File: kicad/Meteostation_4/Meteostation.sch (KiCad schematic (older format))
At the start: 106 parts, among them J1 TxD, J10 GM+, J11 GM-, J12 SWD, J13 SWC, J2 RxD, J3 BME280_SCL, J4 BME280_SDA, J6 +EXT, J7 -EXT, Q1 5N10, Q2 IRLML6346, Q3 Q_NPN_BEC, T1 HY931147C, U1 STM32F103C8Tx, U2 LMR14206, U3 AD8541, Y2 ECS-250-20-33 25MHz

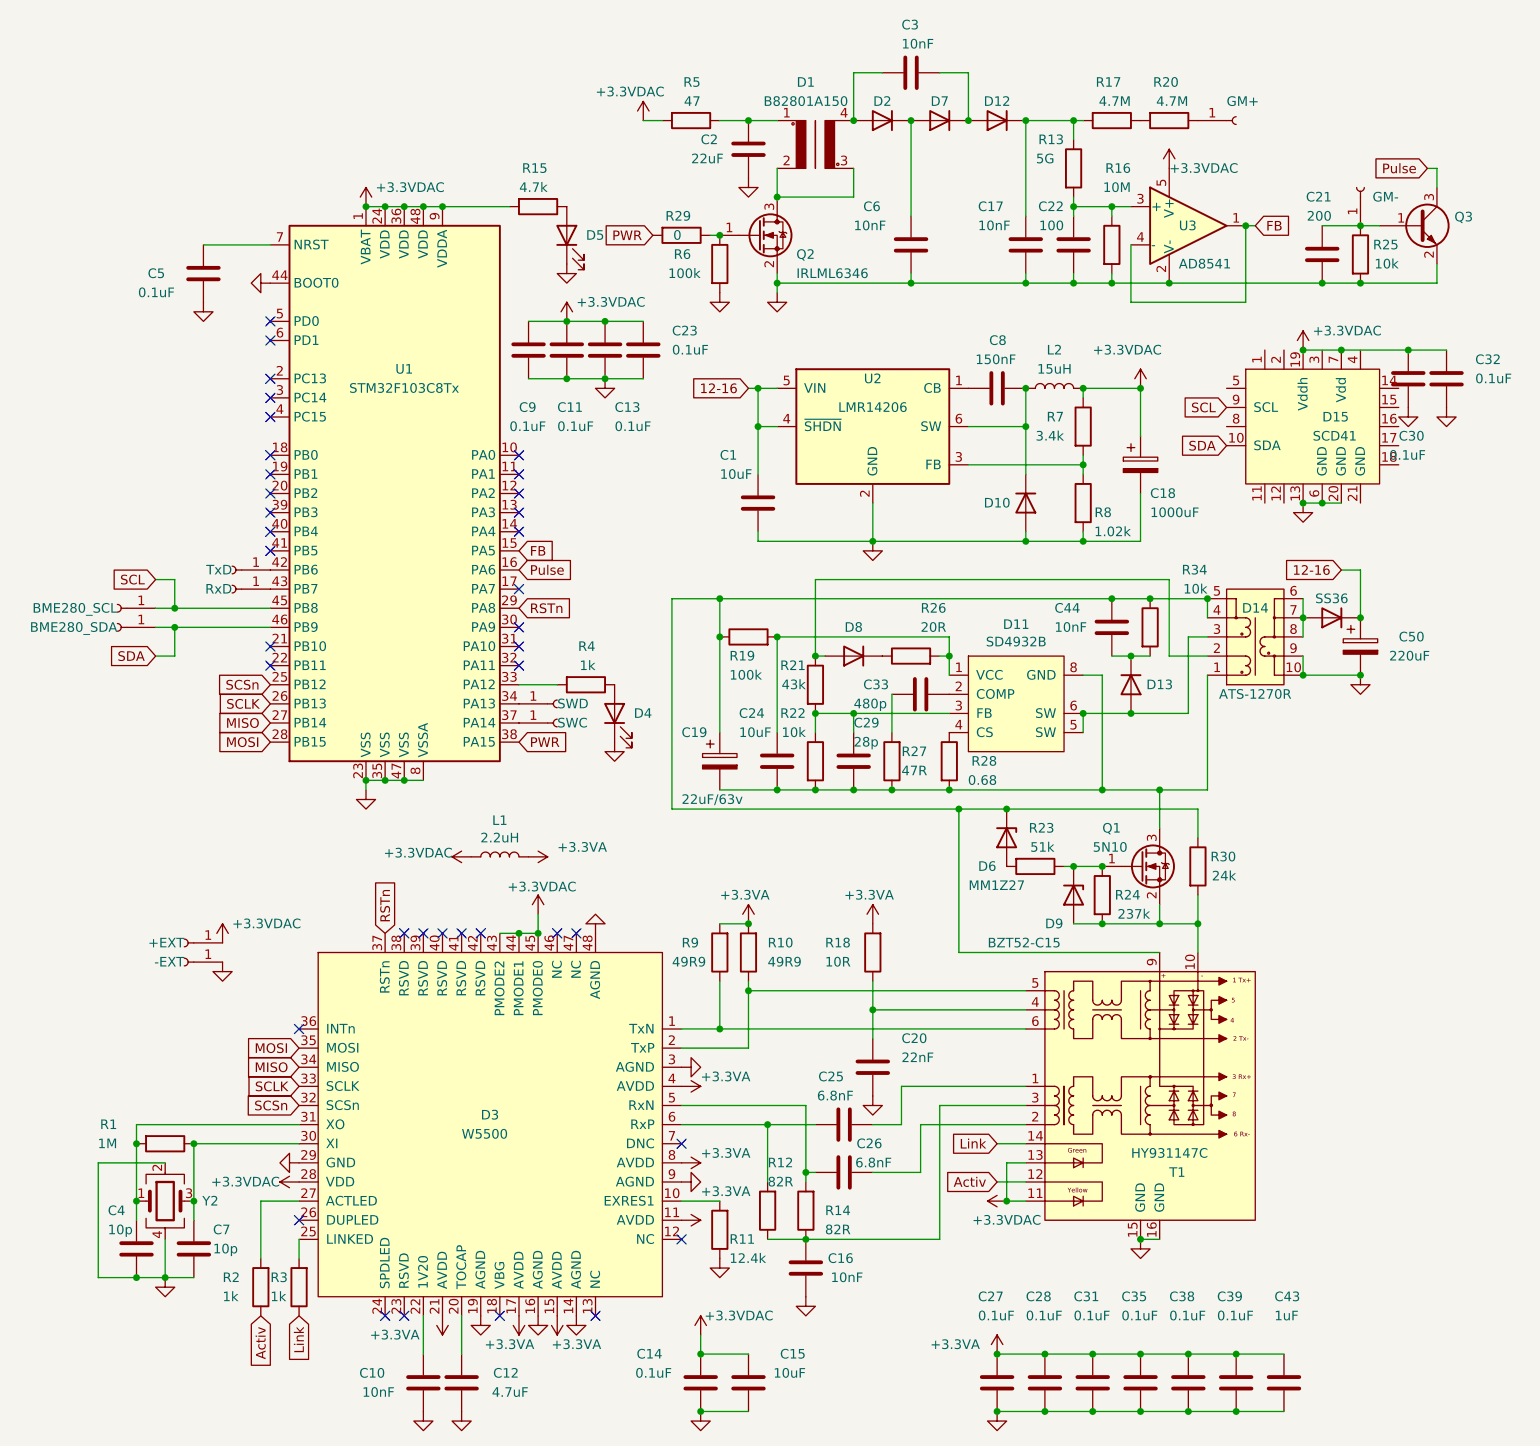
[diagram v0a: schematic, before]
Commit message: изменено:      kicad/Meteostation_4/Meteostation.kicad_pcb 	изменено:      kicad/Meteostation_4/Meteostation.kicad_pcb-bak 	изменено:      kicad/Meteostation_4/Meteostation.sch 	изменено:      kicad/Meteostation_4/Meteostation.sch-bak 	изменено:      kicad/Meteostation_4/fp-info-cache 	изменено:      kicad/Meteostation_4/gerber/Meteostation-job.gbrjob
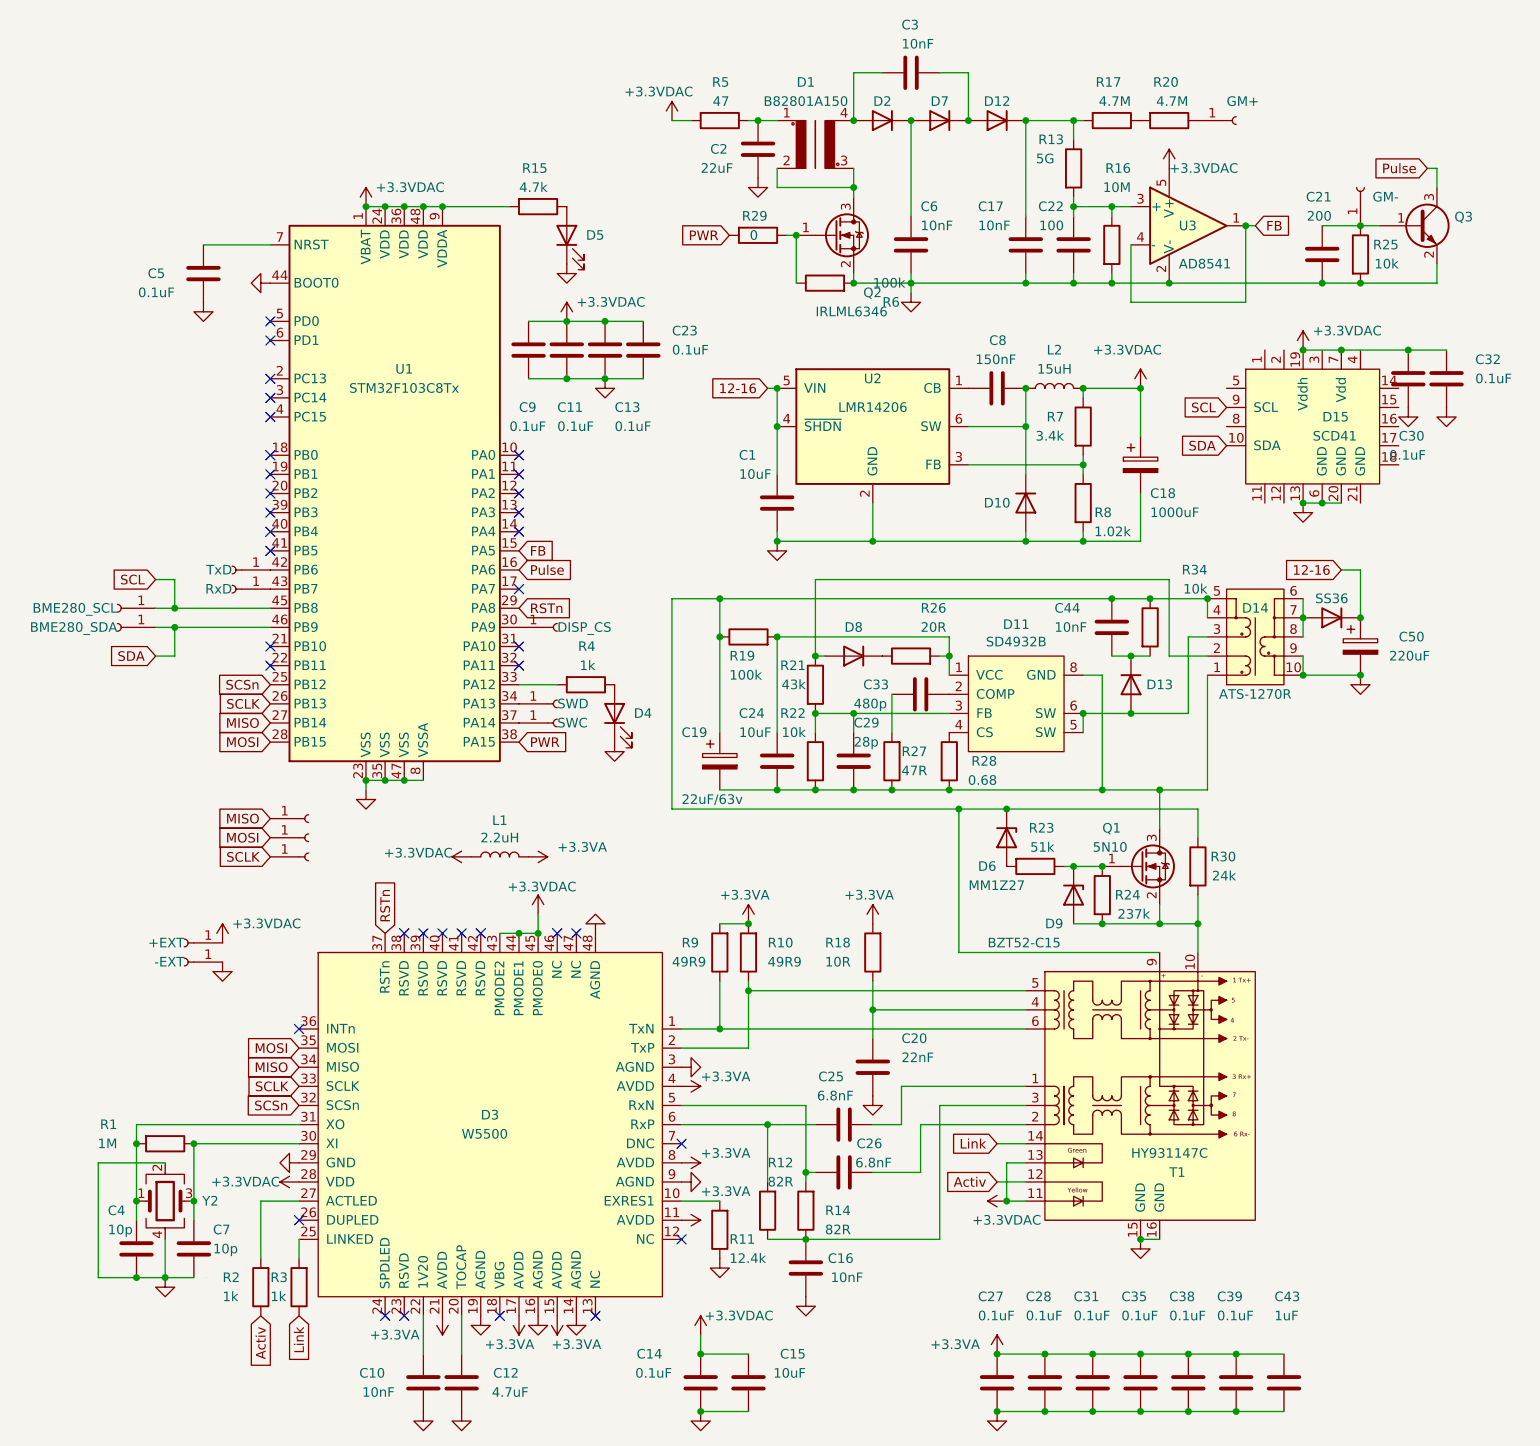
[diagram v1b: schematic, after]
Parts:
- added J14: DISP_CS, My-library:ConnMini, symbol Connector:Conn_01x01_Female
- added J5: miso, My-library:ConnMini, symbol Connector:Conn_01x01_Female
- added J8: mosi, My-library:ConnMini, symbol Connector:Conn_01x01_Female
- added J9: sclk, My-library:ConnMini, symbol Connector:Conn_01x01_Female
- R4: footprint Resistor_SMD:R_0603_1608Metric -> Resistor_SMD:R_0402_1005Metric
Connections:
- net MISO: now also J5.1 (Pin_1)
- net MOSI: now also J8.1 (Pin_1)
- net SCLK: now also J9.1 (Pin_1)
- net at U1.30 (PA9): now also J14.1 (Pin_1)
- no-connect marks 37 -> 36
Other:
- moved on the sheet: C1, C2, Q2, R29, R5, R6
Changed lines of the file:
@@
 F 0 "R4" V 6300 5700 50  0000 R CNN
 F 1 "1k" V 6400 5700 50  0000 R CNN
-F 2 "Resistor_SMD:R_0603_1608Metric" V 6430 5650 50  0001 C CNN
+F 2 "Resistor_SMD:R_0402_1005Metric" V 6430 5650 50  0001 C CNN
 F 3 "~" H 6500 5650 50  0001 C CNN
 	1    6500 5650
@@
 	1    0    0    -1
 $EndComp
-Text GLabel 7350 4100 0    50   Input ~ 0
+Text GLabel 7450 4100 0    50   Input ~ 0
 12-16
 $Comp
@@
 L power:GND #PWR029
 U 1 1 63349FA6
-P 8000 4900
-F 0 "#PWR029" H 8000 4650 50  0001 C CNN
-F 1 "GND" H 8005 4727 50  0001 C CNN
-F 2 "" H 8000 4900 50  0001 C CNN
-F 3 "" H 8000 4900 50  0001 C CNN
-	1    8000 4900
+P 7500 4900
+F 0 "#PWR029" H 7500 4650 50  0001 C CNN
+F 1 "GND" H 7505 4727 50  0001 C CNN
+F 2 "" H 7500 4900 50  0001 C CNN
+F 3 "" H 7500 4900 50  0001 C CNN
+	1    7500 4900
 	1    0    0    -1
 $EndComp
@@
 L Device:C C1
 U 1 1 634777B2
-P 7400 4700
-F 0 "C1" H 7200 4950 50  0000 L CNN
-F 1 "10uF" H 7200 4850 50  0000 L CNN
-F 2 "Capacitor_SMD:C_0805_2012Metric" H 7438 4550 50  0001 C CNN
-F 3 "~" H 7400 4700 50  0001 C CNN
-	1    7400 4700
-	1    0    0    -1
-$EndComp
-Wire Wire Line
-	7400 4100 7500 4100
-Wire Wire Line
-	7500 4300 7400 4300
-Wire Wire Line
-	7400 4300 7400 4100
-Wire Wire Line
-	7400 4300 7400 4550
-Connection ~ 7400 4300
-Wire Wire Line
-	8000 4900 7400 4900
-Wire Wire Line
-	7400 4900 7400 4850
+P 7500 4700
+F 0 "C1" H 7300 4950 50  0000 L CNN
+F 1 "10uF" H 7300 4850 50  0000 L CNN
+F 2 "Capacitor_SMD:C_0805_2012Metric" H 7538 4550 50  0001 C CNN
+F 3 "~" H 7500 4700 50  0001 C CNN
+	1    7500 4700
+	1    0    0    -1
+$EndComp
 $Comp
 L power:GND #PWR013
@@
 $EndComp
 $Comp
-L Transistor_FET:BSS138 Q2
-U 1 1 6364CAE8
-P 7400 3300
-F 0 "Q2" H 7600 3200 50  0000 L CNN
-F 1 "IRLML6346" H 7600 3100 50  0000 L CNN
-F 2 "Package_TO_SOT_SMD:SOT-23" H 7600 3225 50  0001 L CIN
-F 3 "https://www.onsemi.com/pub/Collateral/BSS138-D.PDF" H 7400 3300 50  0001 L CNN
-	1    7400 3300
-	1    0    0    -1
-$EndComp
-$Comp
 L Meteostation-rescue:B82801A1-My_Library D1
 U 1 1 6364FE98
@@
 $EndComp
 Wire Wire Line
-	7500 2950 7500 3100
-Wire Wire Line
-	7500 3100 7900 3100
-Wire Wire Line
-	7900 3100 7900 2950
-Connection ~ 7500 3100
+	7900 3100 7900 3050
 $Comp
 L power:GND #PWR028
 U 1 1 63678BE2
-P 7500 3600
-F 0 "#PWR028" H 7500 3350 50  0001 C CNN
-F 1 "GND" H 7505 3427 50  0001 C CNN
-F 2 "" H 7500 3600 50  0001 C CNN
-F 3 "" H 7500 3600 50  0001 C CNN
-	1    7500 3600
+P 8200 3600
+F 0 "#PWR028" H 8200 3350 50  0001 C CNN
+F 1 "GND" H 8205 3427 50  0001 C CNN
+F 2 "" H 8200 3600 50  0001 C CNN
+F 3 "" H 8200 3600 50  0001 C CNN
+	1    8200 3600
 	1    0    0    -1
 $EndComp
@@
 U 1 1 636874B8
 P 8200 3350
-F 0 "C6" H 7950 3550 50  0000 L CNN
-F 1 "10nF" H 7900 3450 50  0000 L CNN
+F 0 "C6" H 8250 3550 50  0000 L CNN
+F 1 "10nF" H 8250 3450 50  0000 L CNN
 F 2 "Capacitor_SMD:C_1206_3216Metric" H 8238 3200 50  0001 C CNN
 F 3 "~" H 8200 3350 50  0001 C CNN
@@
 $EndComp
 Wire Wire Line
-	7500 3550 7500 3500
-Wire Wire Line
-	7500 3550 7500 3600
-Connection ~ 7500 3550
-Text GLabel 6850 3300 0    50   Input ~ 0
-PWR
+	8200 3550 8200 3600
 $Comp
 L Device:C C2
 U 1 1 63742F99
-P 7350 2850
-F 0 "C2" H 7100 2900 50  0000 L CNN
-F 1 "22uF" H 7050 2800 50  0000 L CNN
-F 2 "Capacitor_SMD:C_0805_2012Metric" H 7388 2700 50  0001 C CNN
-F 3 "~" H 7350 2850 50  0001 C CNN
-	1    7350 2850
-	1    0    0    -1
-$EndComp
-Wire Wire Line
-	7500 2700 7350 2700
+P 7400 2850
+F 0 "C2" H 7150 2850 50  0000 L CNN
+F 1 "22uF" H 7100 2750 50  0000 L CNN
+F 2 "Capacitor_SMD:C_0805_2012Metric" H 7438 2700 50  0001 C CNN
+F 3 "~" H 7400 2850 50  0001 C CNN
+	1    7400 2850
+	1    0    0    -1
+$EndComp
+Wire Wire Line
+	7500 2700 7400 2700
 $Comp
 L power:GND #PWR027
 U 1 1 6374F84D
-P 7350 3000
-F 0 "#PWR027" H 7350 2750 50  0001 C CNN
-F 1 "GND" H 7355 2827 50  0001 C CNN
-F 2 "" H 7350 3000 50  0001 C CNN
-F 3 "" H 7350 3000 50  0001 C CNN
-	1    7350 3000
+P 7400 3000
+F 0 "#PWR027" H 7400 2750 50  0001 C CNN
+F 1 "GND" H 7405 2827 50  0001 C CNN
+F 2 "" H 7400 3000 50  0001 C CNN
+F 3 "" H 7400 3000 50  0001 C CNN
+	1    7400 3000
 	1    0    0    -1
 $EndComp
@@
 L Device:R R5
 U 1 1 63751028
-P 7050 2700
-F 0 "R5" V 6850 2750 50  0000 R CNN
-F 1 "47" V 6950 2750 50  0000 R CNN
-F 2 "Resistor_SMD:R_1206_3216Metric" V 6980 2700 50  0001 C CNN
-F 3 "~" H 7050 2700 50  0001 C CNN
-	1    7050 2700
+P 7200 2700
+F 0 "R5" V 7000 2750 50  0000 R CNN
+F 1 "47" V 7100 2750 50  0000 R CNN
+F 2 "Resistor_SMD:R_1206_3216Metric" V 7130 2700 50  0001 C CNN
+F 3 "~" H 7200 2700 50  0001 C CNN
+	1    7200 2700
 	0    1    1    0
 $EndComp
@@
 L power:+3.3VDAC #PWR023
 U 1 1 63754194
-P 6800 2700
-F 0 "#PWR023" H 6950 2650 50  0001 C CNN
-F 1 "+3.3VDAC" H 6550 2850 50  0000 L CNN
-F 2 "" H 6800 2700 50  0001 C CNN
-F 3 "" H 6800 2700 50  0001 C CNN
-	1    6800 2700
-	1    0    0    -1
-$EndComp
-Wire Wire Line
-	6800 2700 6900 2700
+P 6950 2700
+F 0 "#PWR023" H 7100 2650 50  0001 C CNN
+F 1 "+3.3VDAC" H 6700 2850 50  0000 L CNN
+F 2 "" H 6950 2700 50  0001 C CNN
+F 3 "" H 6950 2700 50  0001 C CNN
+	1    6950 2700
+	1    0    0    -1
+$EndComp
+Wire Wire Line
+	6950 2700 7050 2700
 $Comp
 L Device:R R17
@@
 NoConn ~ 4850 4950
 NoConn ~ 6150 5150
-NoConn ~ 6150 5350
 NoConn ~ 6150 5450
 NoConn ~ 6150 5550
@@
 	10950 3450 10950 3550
 Wire Wire Line
-	7350 4100 7400 4100
-Connection ~ 7400 4100
-Wire Wire Line
 	10900 2950 10950 2950
 Wire Wire Line
@@
 Wire Wire Line
 	9250 3200 9250 3150
-Wire Wire Line
-	7500 3550 8200 3550
 Connection ~ 9250 3150
 Wire Wire Line
@@
 Wire Wire Line
 	8200 3550 8800 3550
-Connection ~ 7350 2700
-Wire Wire Line
-	7350 2700 7200 2700
 Wire Wire Line
 	7650 7850 7650 8200
@@
 	7700 5100 9550 5100
 $Comp
-L Device:R R6
-U 1 1 634FB19F
-P 7200 3450
-F 0 "R6" H 7050 3500 50  0000 R CNN
-F 1 "100k" H 7100 3400 50  0000 R CNN
-F 2 "Resistor_SMD:R_0603_1608Metric" V 7130 3450 50  0001 C CNN
-F 3 "~" H 7200 3450 50  0001 C CNN
-	1    7200 3450
-	1    0    0    -1
-$EndComp
-$Comp
-L power:GND #PWR043
-U 1 1 63505702
-P 7200 3600
-F 0 "#PWR043" H 7200 3350 50  0001 C CNN
-F 1 "GND" H 7205 3427 50  0001 C CNN
-F 2 "" H 7200 3600 50  0001 C CNN
-F 3 "" H 7200 3600 50  0001 C CNN
-	1    7200 3600
-	1    0    0    -1
-$EndComp
-$Comp
 L Device:R R16
 U 1 1 636A0C6A
@@
 Wire Wire Line
 	10800 3900 11000 3900
+Wire Wire Line
+	7550 3300 7600 3300
 $Comp
 L Device:R R29
 U 1 1 635E067E
-P 7000 3300
-F 0 "R29" V 6900 3350 50  0000 R CNN
-F 1 "0" V 7000 3300 50  0000 R CNN
-F 2 "Resistor_SMD:R_1206_3216Metric" V 6930 3300 50  0001 C CNN
-F 3 "~" H 7000 3300 50  0001 C CNN
-	1    7000 3300
+P 7400 3300
+F 0 "R29" V 7300 3350 50  0000 R CNN
+F 1 "0" V 7400 3300 50  0000 R CNN
+F 2 "Resistor_SMD:R_1206_3216Metric" V 7330 3300 50  0001 C CNN
+F 3 "~" H 7400 3300 50  0001 C CNN
+	1    7400 3300
 	0    1    1    0
 $EndComp
-Wire Wire Line
-	7150 3300 7200 3300
-Connection ~ 7200 3300
+$Comp
+L Device:R R6
+U 1 1 634FB19F
+P 7750 3550
+F 0 "R6" V 7650 3250 50  0000 R CNN
+F 1 "100k" V 7750 3300 50  0000 R CNN
+F 2 "Resistor_SMD:R_0603_1608Metric" V 7680 3550 50  0001 C CNN
+F 3 "~" H 7750 3550 50  0001 C CNN
+	1    7750 3550
+	0    -1   -1   0
+$EndComp
+Text GLabel 7250 3300 0    50   Input ~ 0
+PWR
+$Comp
+L Transistor_FET:BSS138 Q2
+U 1 1 6364CAE8
+P 7800 3300
+F 0 "Q2" H 7950 3000 50  0000 L CNN
+F 1 "IRLML6346" H 7700 2900 50  0000 L CNN
+F 2 "Package_TO_SOT_SMD:SOT-23" H 8000 3225 50  0001 L CIN
+F 3 "https://www.onsemi.com/pub/Collateral/BSS138-D.PDF" H 7800 3300 50  0001 L CNN
+	1    7800 3300
+	1    0    0    -1
+$EndComp
+Wire Wire Line
+	7900 3500 7900 3550
+Wire Wire Line
+	7900 3550 8200 3550
+Connection ~ 7900 3550
+Wire Wire Line
+	7600 3550 7600 3300
+Connection ~ 7600 3300
+Wire Wire Line
+	7350 2700 7400 2700
+Connection ~ 7400 2700
+Wire Wire Line
+	7500 2950 7500 3050
+Wire Wire Line
+	7500 3050 7900 3050
+Connection ~ 7900 3050
+Wire Wire Line
+	7900 3050 7900 2950
+$Comp
+L Connector:Conn_01x01_Female J14
+U 1 1 6380E229
+P 6350 5350
+F 0 "J14" H 6600 5350 50  0001 C CNN
+F 1 "DISP_CS" H 6350 5350 50  0000 L CNN
+F 2 "My-library:ConnMini" H 6350 5350 50  0001 C CNN
+F 3 "~" H 6350 5350 50  0001 C CNN
+	1    6350 5350
+	1    0    0    -1
+$EndComp
+$Comp
+L Connector:Conn_01x01_Female J5
+U 1 1 638107F7
+P 5050 6350
+F 0 "J5" H 5300 6350 50  0001 C CNN
+F 1 "miso" H 5050 6350 50  0001 L CNN
+F 2 "My-library:ConnMini" H 5050 6350 50  0001 C CNN
+F 3 "~" H 5050 6350 50  0001 C CNN
+	1    5050 6350
+	1    0    0    -1
+$EndComp
+$Comp
+L Connector:Conn_01x01_Female J8
+U 1 1 6381117F
+P 5050 6450
+F 0 "J8" H 5300 6450 50  0001 C CNN
+F 1 "mosi" H 5050 6450 50  0001 L CNN
+F 2 "My-library:ConnMini" H 5050 6450 50  0001 C CNN
+F 3 "~" H 5050 6450 50  0001 C CNN
+	1    5050 6450
+	1    0    0    -1
+$EndComp
+$Comp
+L Connector:Conn_01x01_Female J9
+U 1 1 63811811
+P 5050 6550
+F 0 "J9" H 5300 6550 50  0001 C CNN
+F 1 "sclk" H 5050 6550 50  0001 L CNN
+F 2 "My-library:ConnMini" H 5050 6550 50  0001 C CNN
+F 3 "~" H 5050 6550 50  0001 C CNN
+	1    5050 6550
+	1    0    0    -1
+$EndComp
+Text GLabel 4850 6350 0    50   Input ~ 0
+MISO
+Text GLabel 4850 6450 0    50   Input ~ 0
+MOSI
+Text GLabel 4850 6550 0    50   Input ~ 0
+SCLK
+Wire Wire Line
+	7500 4550 7500 4300
+Connection ~ 7500 4300
+Wire Wire Line
+	7500 4300 7500 4100
+Wire Wire Line
+	8000 4900 7500 4900
+Wire Wire Line
+	7500 4900 7500 4850
+Connection ~ 7500 4900
+Wire Wire Line
+	7450 4100 7500 4100
+Connection ~ 7500 4100
 $EndSCHEMATC

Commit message: изменено:      kicad/Meteostation_4/Meteostation.sch 	изменено:      kicad/Meteostation_4/Meteostation.sch-bak 	изменено:      stm32cubeide/Meteostation/.mxproject 	изменено:      stm32cubeide/Meteostation/.settings/language.settings.xml 	изменено:      stm32cubeide/Meteostation/Core/Inc/main.h 	изменено:      stm32cubeide/Meteostation/Core/Src/main.c 	изменено:      stm32cubeide/Meteostation/Meteostation.ioc 	изменено:      stm32cubeide/Meteostation/Release/Core/Src/BME280.d 	изменено:      stm32cubeide/Meteostation/Release/Core/Src/main.d 	изменено:      stm32cubeide/Meteostation/Release/Core/Src/main.o 	изменено:      stm32cubeide/Meteostation/Release/Core/Src/main.su 	изменено:      stm32cubeide/Meteostation/Release/Core/Src/stm32f1xx_hal_msp.d 	изменено:      stm32cubeide/Meteostation/Release/Core/Src/stm32f1xx_it.d 	изменено:      stm32cubeide/Meteostation/Release/Core/Src/stm32f1xx_it.o 	изменено:      stm32cubeide/Meteostation/Release/Meteostation.bin 	изменено:      stm32cubeide/Meteostation/Release/Meteostation.elf 	изменено:      stm32cubeide/Meteostation/Release/Meteostation.hex 	изменено:      stm32cubeide/Meteostation/Release/Meteostation.list 	изменено:      stm32cubeide/Meteostation/Release/Meteostation.map 	изменено:      stm32cubeide/Meteostation/Release/makefile
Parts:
- D10: value SS56 -> SS56, VS10MQ060-M3/5
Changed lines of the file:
@@
 P 8800 4700
 F 0 "D10" V 8800 4550 50  0000 C CNN
-F 1 "SS56" H 8700 4550 50  0001 C CNN
+F 1 "SS56, VS10MQ060-M3/5" H 8700 4550 50  0001 C CNN
 F 2 "Diode_SMD:D_SMA" H 8800 4700 50  0001 C CNN
 F 3 "~" H 8800 4700 50  0001 C CNN
